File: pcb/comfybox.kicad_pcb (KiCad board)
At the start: 2 copper layers, 242 x 138 mm, 20 parts, among them K1 SW_CHOC, K2 SW_CHOC, K3 SW_CHOC, K4 SW_CHOC, P1 SW_CHOC, P2 SW_CHOC, P3 SW_CHOC, P4 SW_CHOC

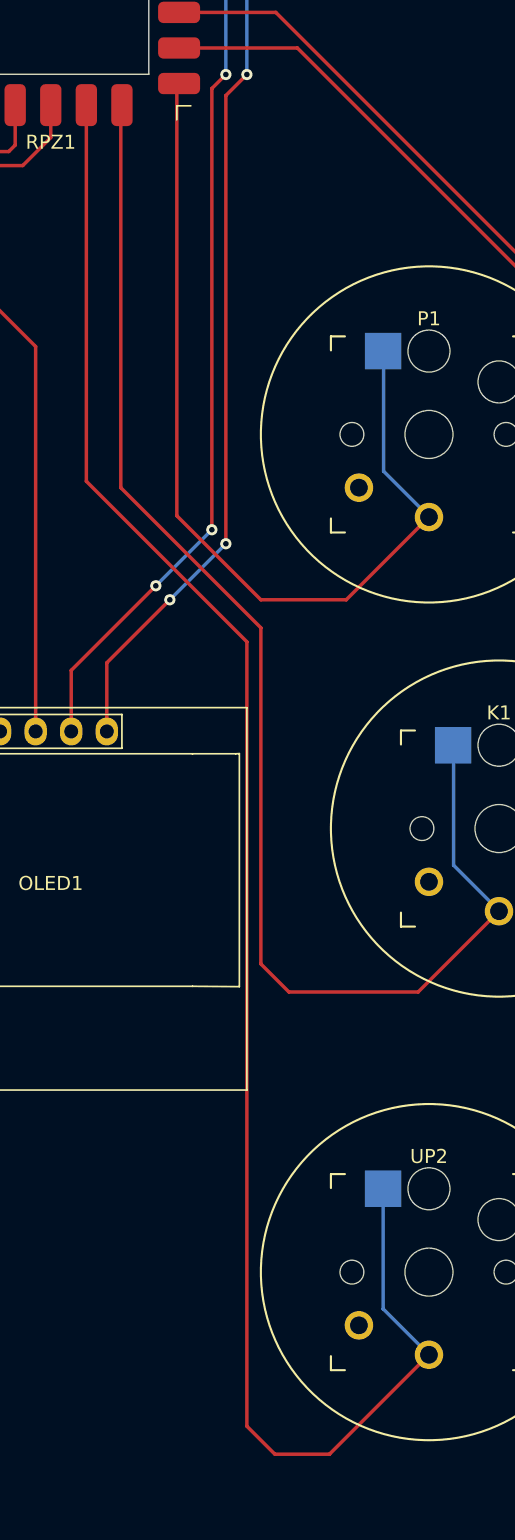
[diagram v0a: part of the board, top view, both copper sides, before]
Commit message: adjust tracing
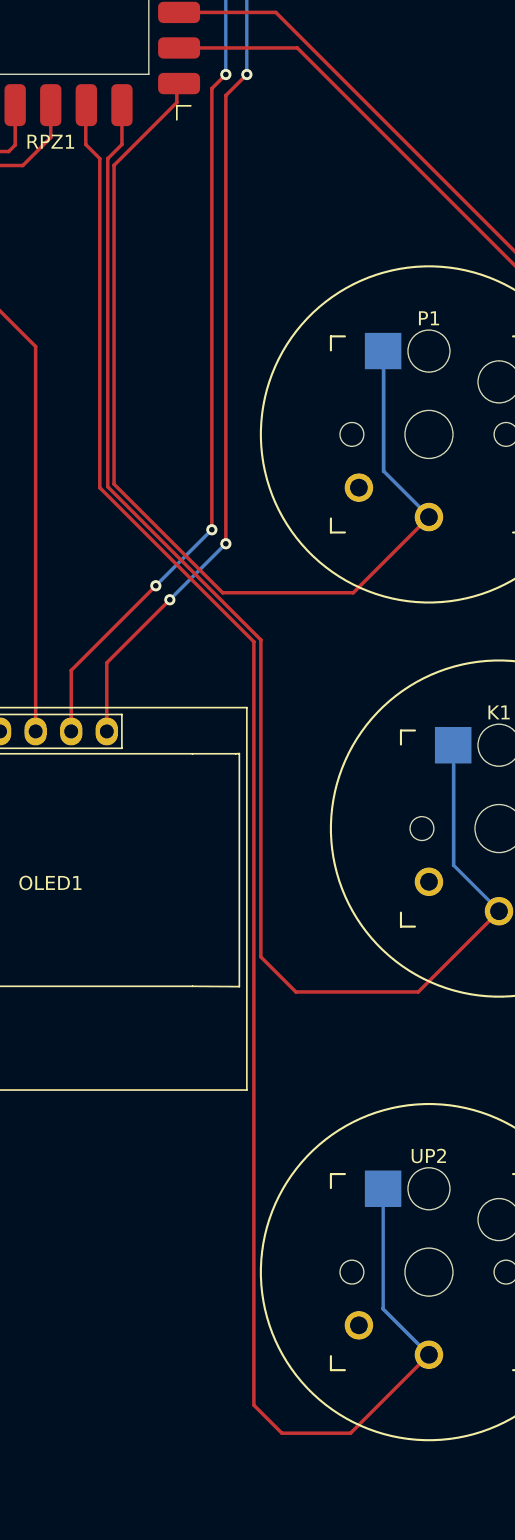
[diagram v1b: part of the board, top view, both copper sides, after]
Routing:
- net P1: track 67.1 -> 71.7 mm
- net UP R: track 129.0 -> 126.7 mm
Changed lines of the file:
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@@
   (gr_line (start 142 23) (end 257 23) (layer "Edge.Cuts") (width 0.1))
   (gr_line (start 128 44.485516) (end 128 23) (layer "Edge.Cuts") (width 0.1))
-  (segment (start 144 76) (end 144 45.305516) (width 0.25) (layer "F.Cu") (net 1))
-  (segment (start 150 82) (end 144 76) (width 0.25) (layer "F.Cu") (net 1))
-  (segment (start 156.095571 82) (end 150 82) (width 0.25) (layer "F.Cu") (net 1))
+  (segment (start 147.272792 81.5) (end 139.518198 73.745406) (width 0.25) (layer "F.Cu") (net 1))
+  (segment (start 144 46.5) (end 144 45.305516) (width 0.25) (layer "F.Cu") (net 1))
   (segment (start 144 45.305516) (end 144.16 45.145516) (width 0.25) (layer "F.Cu") (net 1))
-  (segment (start 162.00027 76.095301) (end 156.095571 82) (width 0.25) (layer "F.Cu") (net 1))
+  (segment (start 139.518198 50.981802) (end 144 46.5) (width 0.25) (layer "F.Cu") (net 1))
+  (segment (start 156.595571 81.5) (end 147.272792 81.5) (width 0.25) (layer "F.Cu") (net 1))
+  (segment (start 162.00027 76.095301) (end 156.595571 81.5) (width 0.25) (layer "F.Cu") (net 1))
+  (segment (start 139.518198 73.745406) (end 139.518198 50.981802) (width 0.25) (layer "F.Cu") (net 1))
   (segment (start 158.76027 72.820301) (end 162.03527 76.095301) (width 0.25) (layer "B.Cu") (net 1))
   (segment (start 158.76027 64.245301) (end 158.76027 72.820301) (width 0.25) (layer "B.Cu") (net 1))
@@
   (segment (start 236.631082 46.172382) (end 239.906082 49.447382) (width 0.25) (layer "B.Cu") (net 5))
   (segment (start 236.631082 37.597382) (end 236.631082 46.172382) (width 0.25) (layer "B.Cu") (net 5))
-  (segment (start 150 84) (end 140 74) (width 0.25) (layer "F.Cu") (net 6))
-  (segment (start 140 74) (end 140 46.765516) (width 0.25) (layer "F.Cu") (net 6))
-  (segment (start 140 46.765516) (end 140.08 46.685516) (width 0.25) (layer "F.Cu") (net 6))
-  (segment (start 152 110) (end 150 108) (width 0.25) (layer "F.Cu") (net 6))
+  (segment (start 150 84.863604) (end 139.068198 73.931802) (width 0.25) (layer "F.Cu") (net 6))
+  (segment (start 152.5 110) (end 150 107.5) (width 0.25) (layer "F.Cu") (net 6))
   (segment (start 167.00027 104.233869) (end 161.234139 110) (width 0.25) (layer "F.Cu") (net 6))
-  (segment (start 161.234139 110) (end 152 110) (width 0.25) (layer "F.Cu") (net 6))
-  (segment (start 150 108) (end 150 84) (width 0.25) (layer "F.Cu") (net 6))
+  (segment (start 139.068198 50.511802) (end 140.08 49.5) (width 0.25) (layer "F.Cu") (net 6))
+  (segment (start 161.234139 110) (end 152.5 110) (width 0.25) (layer "F.Cu") (net 6))
+  (segment (start 150 107.5) (end 150 84.863604) (width 0.25) (layer "F.Cu") (net 6))
+  (segment (start 140.08 49.5) (end 140.08 46.685516) (width 0.25) (layer "F.Cu") (net 6))
+  (segment (start 139.068198 73.931802) (end 139.068198 50.5) (width 0.25) (layer "F.Cu") (net 6))
   (segment (start 163.76027 100.958869) (end 167.03527 104.233869) (width 0.25) (layer "B.Cu") (net 6))
   (segment (start 163.76027 92.383869) (end 163.76027 100.958869) (width 0.25) (layer "B.Cu") (net 6))
@@
   (segment (start 103.725 132.625) (end 107 135.9) (width 0.25) (layer "B.Cu") (net 13))
   (segment (start 103.725 124.05) (end 103.725 132.625) (width 0.25) (layer "B.Cu") (net 13))
-  (segment (start 162 135.9) (end 154.9 143) (width 0.25) (layer "F.Cu") (net 14))
-  (segment (start 149 85) (end 137.54 73.54) (width 0.25) (layer "F.Cu") (net 14))
-  (segment (start 154.9 143) (end 151 143) (width 0.25) (layer "F.Cu") (net 14))
-  (segment (start 137.54 73.54) (end 137.54 46.685516) (width 0.25) (layer "F.Cu") (net 14))
-  (segment (start 149 141) (end 149 85) (width 0.25) (layer "F.Cu") (net 14))
-  (segment (start 151 143) (end 149 141) (width 0.25) (layer "F.Cu") (net 14))
+  (segment (start 149.5 139.5) (end 149.5 85) (width 0.25) (layer "F.Cu") (net 14))
+  (segment (start 137.5 46.725516) (end 137.54 46.685516) (width 0.25) (layer "F.Cu") (net 14))
+  (segment (start 162 135.9) (end 156.4 141.5) (width 0.25) (layer "F.Cu") (net 14))
+  (segment (start 149.5 85) (end 138.5 74) (width 0.25) (layer "F.Cu") (net 14))
+  (segment (start 138.5 74) (end 138.5 50.5) (width 0.25) (layer "F.Cu") (net 14))
+  (segment (start 156.4 141.5) (end 151.5 141.5) (width 0.25) (layer "F.Cu") (net 14))
+  (segment (start 138.5 50.5) (end 137.5 49.5) (width 0.25) (layer "F.Cu") (net 14))
+  (segment (start 151.5 141.5) (end 149.5 139.5) (width 0.25) (layer "F.Cu") (net 14))
+  (segment (start 137.5 49.5) (end 137.5 46.725516) (width 0.25) (layer "F.Cu") (net 14))
   (segment (start 158.725 132.625) (end 162 135.9) (width 0.25) (layer "B.Cu") (net 14))
   (segment (start 158.725 124.05) (end 158.725 132.625) (width 0.25) (layer "B.Cu") (net 14))
